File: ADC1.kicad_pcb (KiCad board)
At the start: 2 copper layers, 21 parts, among them U8 MCP6004

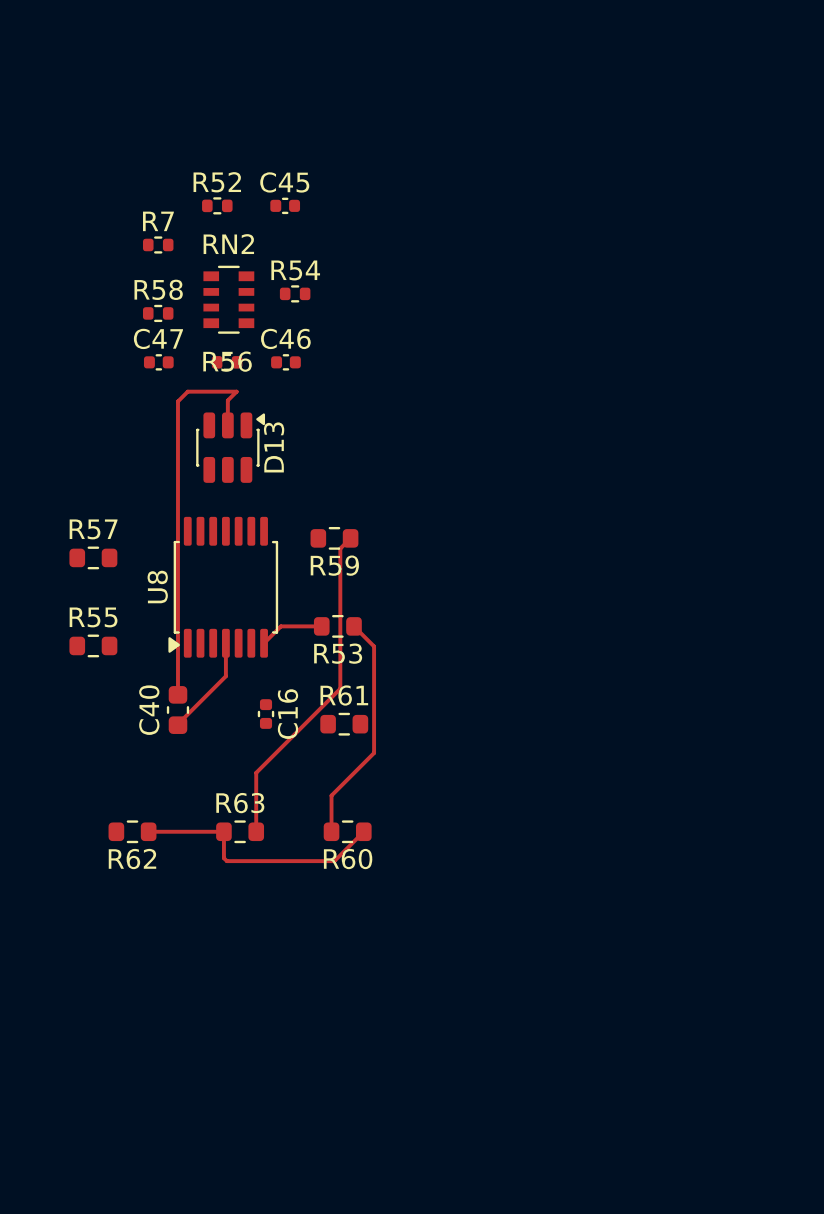
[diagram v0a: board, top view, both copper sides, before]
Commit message: haciendo el pcb
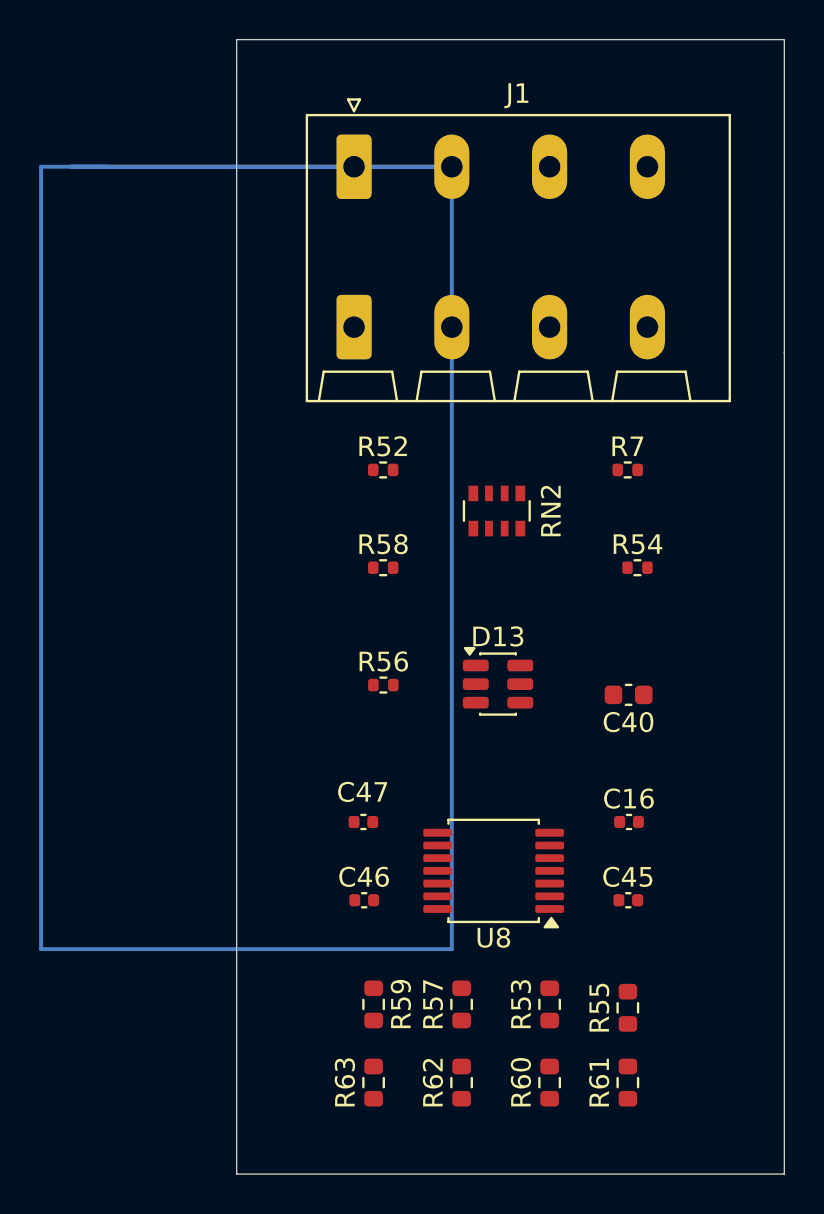
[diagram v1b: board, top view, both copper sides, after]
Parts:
- added J1: Conn_01x04_Shielded, Connector_Phoenix_SPT:PhoenixContact_SPT_2.5_4-H-5.0-EX_1x04_P5.0mm_Horizontal, F.Cu at (111.0, 85.5)
- moved C45 39.6 mm to (125.0, 123.0)
- moved R55 33.0 mm to (125.0, 128.5), turned to 90 degrees
- moved R57 29.6 mm to (116.5, 128.3), turned to 90 degrees
- moved C46 27.8 mm to (111.5, 123.0)
- moved R7 26.6 mm to (125.0, 101.0)
- moved C47 25.7 mm to (111.5, 119.0)
- moved R59 23.9 mm to (112.0, 128.3), turned to -90 degrees
- moved R61 23.4 mm to (125.0, 132.3), turned to 90 degrees
- moved C40 23.1 mm to (125.0, 112.5), turned to 180 degrees
- moved R54 22.4 mm to (125.5, 106.0)
- moved R53 22.2 mm to (121.0, 128.3), turned to 90 degrees
- moved R62 21.2 mm to (116.5, 132.3), turned to 90 degrees
- moved U8 19.9 mm to (118.1, 121.5), turned to 180 degrees
- moved C16 19.4 mm to (125.1, 119.0), turned to 0 degrees
- moved D13 18.4 mm to (118.4, 112.0), turned to 0 degrees
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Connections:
- net /AV6 renamed Net-(J1-Pin_1)
- net /AV7 renamed Net-(J1-Pin_2)
- net /AV8 renamed Net-(J1-Pin_3)
- net /AV9 renamed Net-(J1-Pin_4)
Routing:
- net GND: track 20.1 -> 0.00 mm
- net /AV6_MCU: track 17.0 -> 0.00 mm
- net /AGND: track 13.0 -> 0.00 mm
- net /AV9_MCU: track 11.8 -> 0.00 mm
- net /5V: track 5.15 -> 0.00 mm
- net Net-(U8B--): track 3.31 -> 0.00 mm
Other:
- board outline added: 28 x 58 mm
